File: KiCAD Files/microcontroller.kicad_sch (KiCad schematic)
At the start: 49 parts, among them IC5 AZ1117IH-3.3TRG1, J3 TSW-103-14-S-D, J4 TSW-103-14-S-D, J7 TSW-105-05-F-S, U1 STM32H7A3RGTx, Y1 ABM8G-48.000MHZ-18-D2Y-T

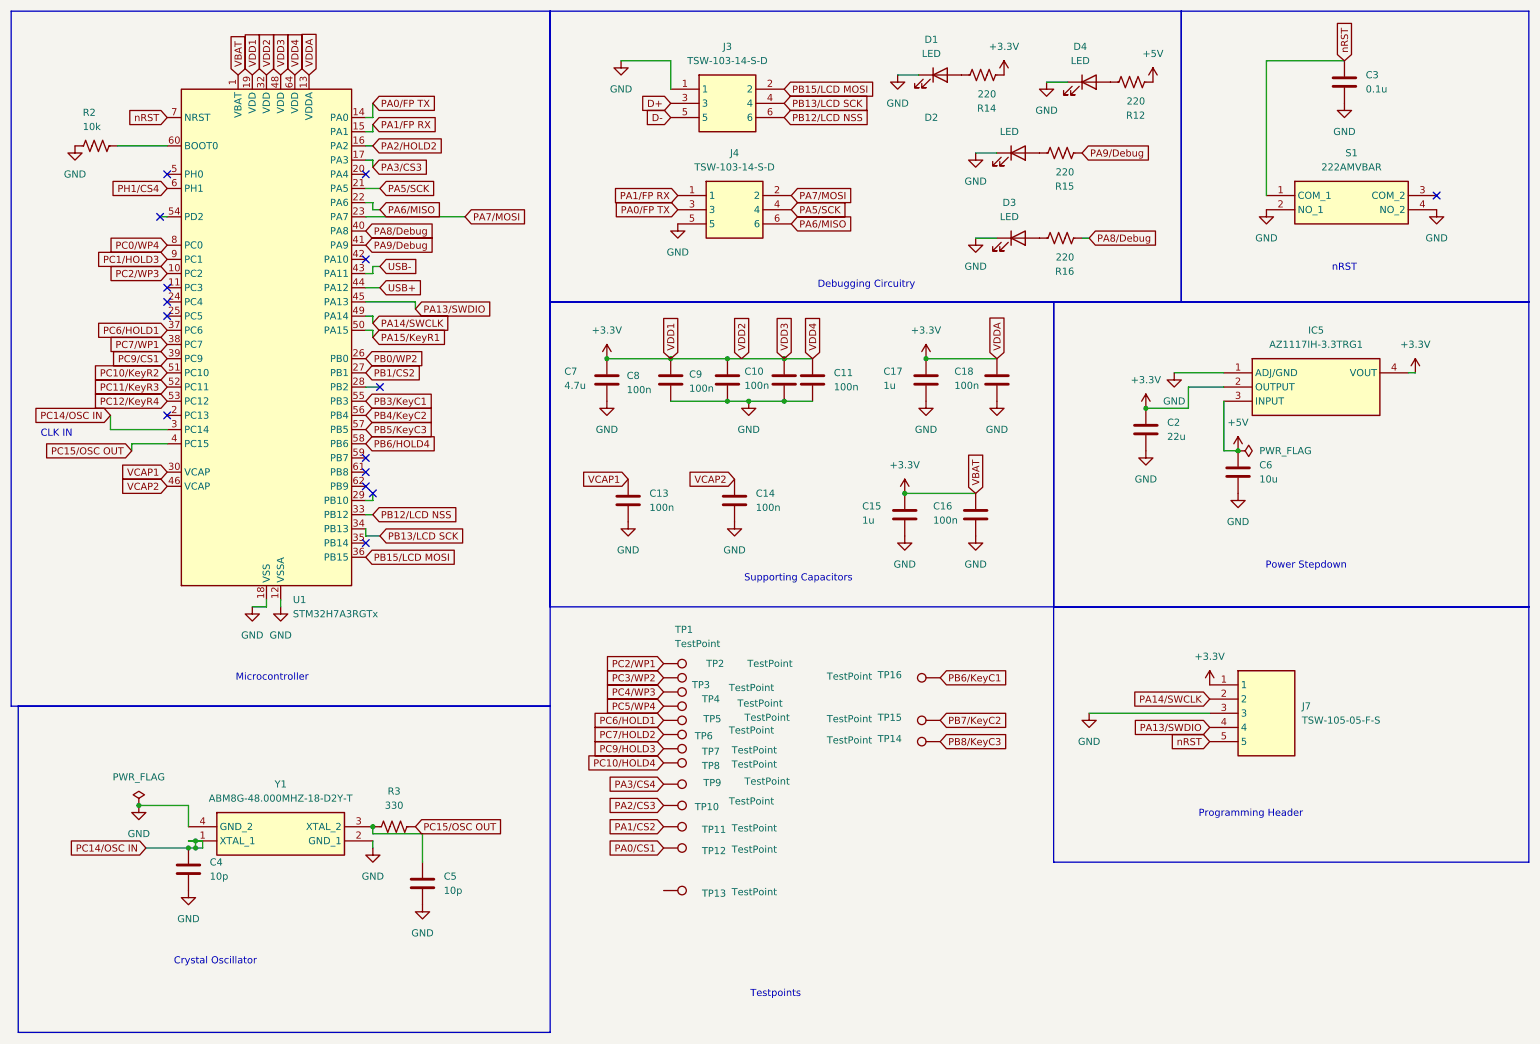
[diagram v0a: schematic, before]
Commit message: finalized 99% of pcb
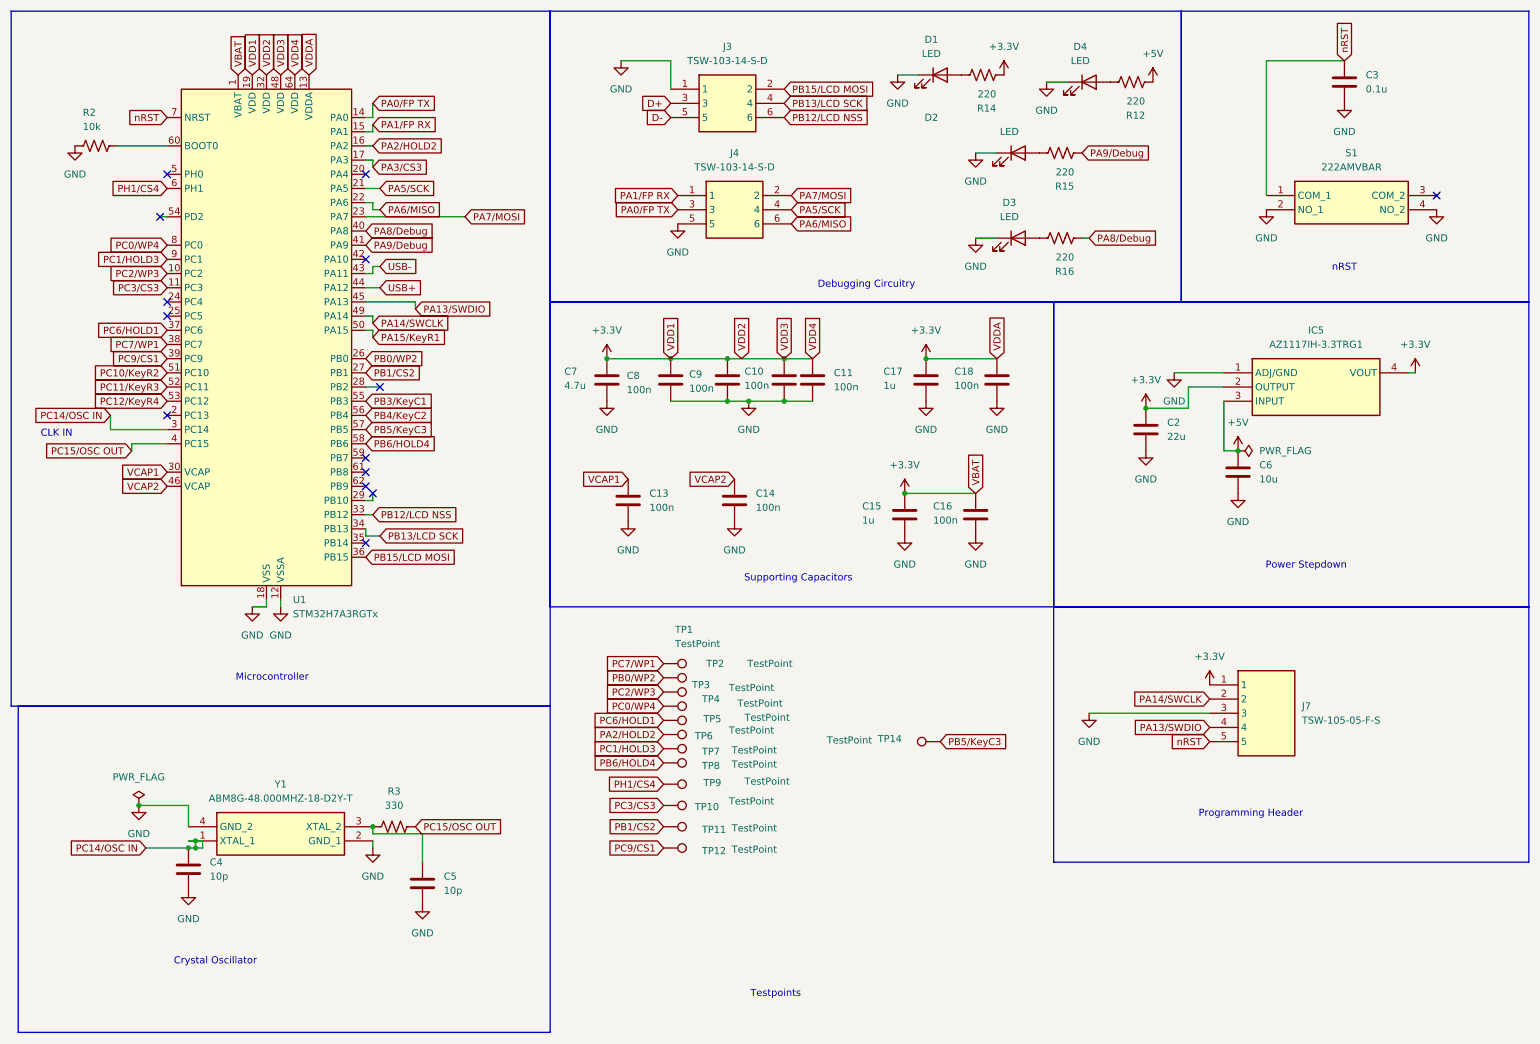
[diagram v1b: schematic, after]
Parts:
- removed TP13, TP15, TP16: TestPoint, TestPoint:TestPoint_THTPad_D1.5mm_Drill0.7mm, symbol Connector:TestPoint
- TP1, TP10, TP11, TP12, TP14, TP2, TP3, TP4, TP5, TP6, TP7, TP8, TP9: footprint TestPoint:TestPoint_THTPad_D1.5mm_Drill0.7mm -> TestPoint:TestPoint_THTPad_D1.0mm_Drill0.5mm
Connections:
- net PA0/CS1 is gone; now on net PC9/CS1: TP12.1
- net PA1/CS2 is gone; now on net PB1/CS2: TP11.1
- net PA2/CS3 is gone; now on net PC3/CS3: TP10.1
- net PA3/CS4 is gone; now on net PH1/CS4: TP9.1
- net PB8/KeyC3 is gone; now on net PB5/KeyC3: TP14.1
- net PC10/HOLD4 is gone; now on net PB6/HOLD4: TP8.1
- net PC2/WP1 is gone; now on net PC7/WP1: TP1.1
- net PC3/WP2 is gone; now on net PB0/WP2: TP2.1
- net PC4/WP3 is gone; now on net PC2/WP3: TP3.1
- net PC5/WP4 is gone; now on net PC0/WP4: TP4.1
- net PC7/HOLD2 is gone; now on net PA2/HOLD2: TP6.1
- net PC9/HOLD3 is gone; now on net PC1/HOLD3: TP7.1
- net PC3/CS3: now reaches U1.11 (PC3)
- no-connect marks 15 -> 14

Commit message: updated files with 3d models
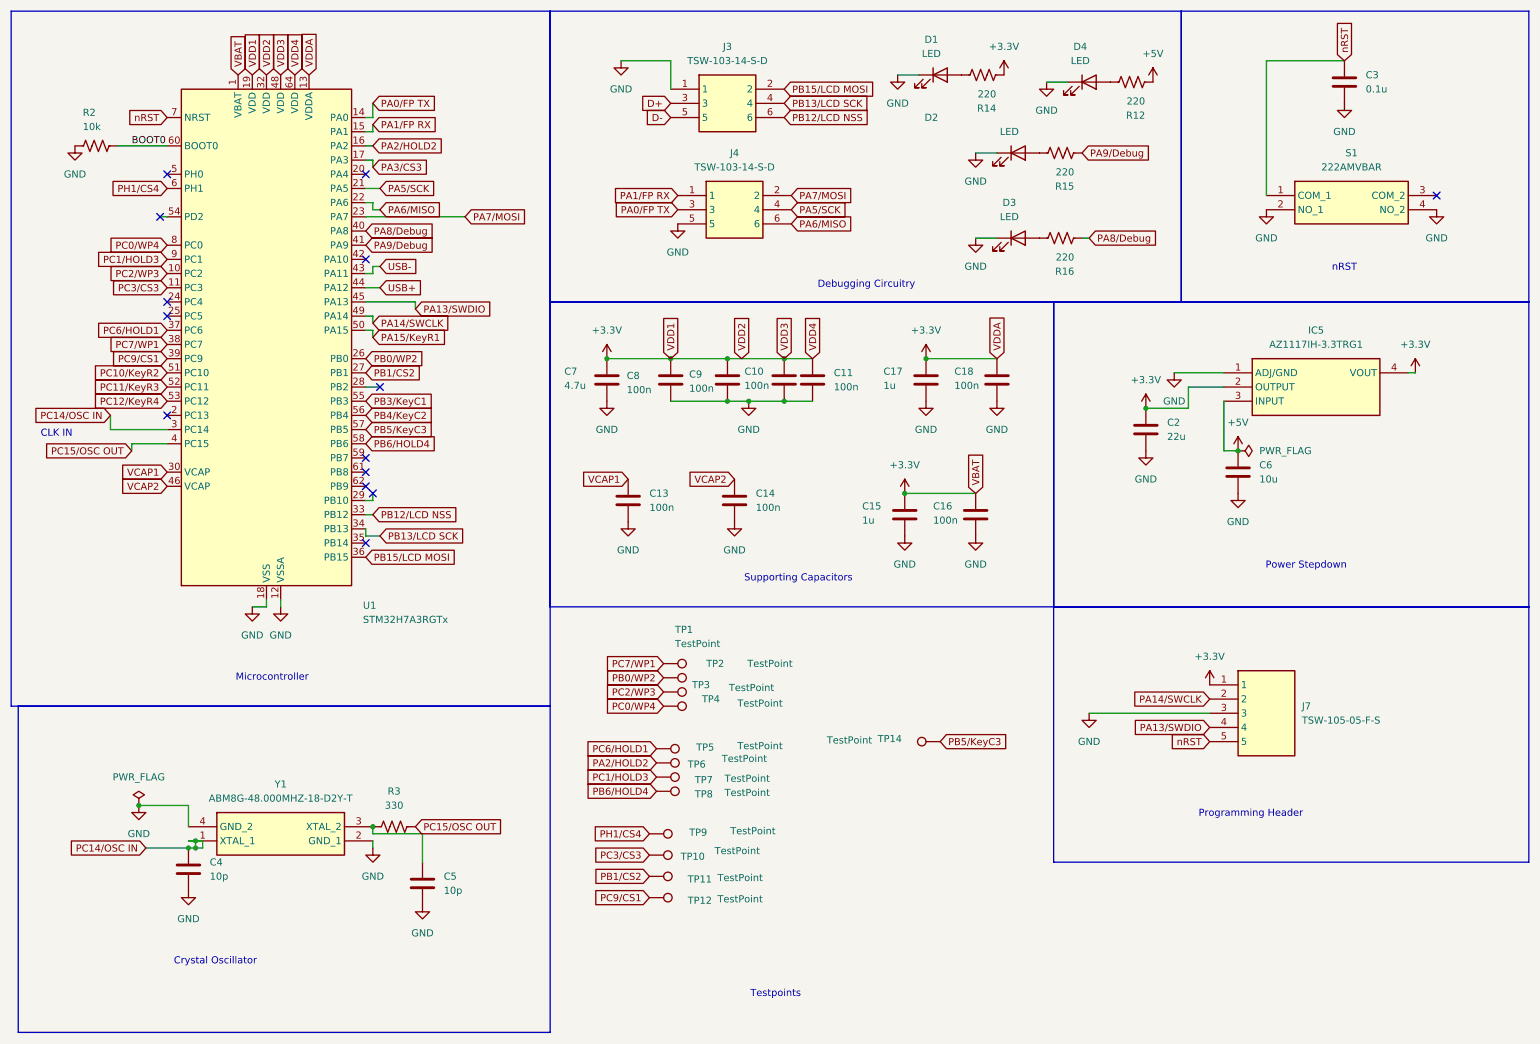
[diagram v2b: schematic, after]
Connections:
- net BOOT0: now reaches R2.1, U1.60 (BOOT0)
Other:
- moved on the sheet: TP10, TP11, TP12, TP5, TP6, TP7, TP8, TP9
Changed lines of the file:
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@@
 		)
 	)
+	(label "BOOT0"
+		(at 34.29 36.83 0)
+		(effects
+			(font
+				(size 1.27 1.27)
+			)
+			(justify left bottom)
+		)
+	)
 	(global_label "PC6{slash}HOLD1"
 		(shape input)
@@
 	(global_label "PC6{slash}HOLD1"
 		(shape input)
-		(at 129.54 139.7 180)
+		(at 128.27 144.78 180)
 		(fields_autoplaced yes)
 		(effects
@@
 		)
 		(property "Intersheetrefs" "${INTERSHEET_REFS}"
-			(at 115.3062 139.7 0)
+			(at 114.0362 144.78 0)
 			(effects
 				(font
@@
 	(global_label "PB1{slash}CS2"
 		(shape input)
-		(at 129.54 158.75 180)
+		(at 127 167.64 180)
 		(fields_autoplaced yes)
 		(effects
@@
 		)
 		(property "Intersheetrefs" "${INTERSHEET_REFS}"
-			(at 117.7858 158.75 0)
+			(at 115.2458 167.64 0)
 			(effects
 				(font
@@
 	(global_label "PH1{slash}CS4"
 		(shape input)
-		(at 129.54 151.13 180)
+		(at 127 160.02 180)
 		(fields_autoplaced yes)
 		(effects
@@
 		)
 		(property "Intersheetrefs" "${INTERSHEET_REFS}"
-			(at 117.7253 151.13 0)
+			(at 115.1853 160.02 0)
 			(effects
 				(font
@@
 	(global_label "PC1{slash}HOLD3"
 		(shape input)
-		(at 129.54 144.78 180)
+		(at 128.27 149.86 180)
 		(fields_autoplaced yes)
 		(effects
@@
 		)
 		(property "Intersheetrefs" "${INTERSHEET_REFS}"
-			(at 115.3062 144.78 0)
+			(at 114.0362 149.86 0)
 			(effects
 				(font
@@
 	(global_label "PB6{slash}HOLD4"
 		(shape input)
-		(at 129.54 147.32 180)
+		(at 128.27 152.4 180)
 		(fields_autoplaced yes)
 		(effects
@@
 		)
 		(property "Intersheetrefs" "${INTERSHEET_REFS}"
-			(at 115.3062 147.32 0)
+			(at 114.0362 152.4 0)
 			(effects
 				(font
@@
 	(global_label "PA2{slash}HOLD2"
 		(shape input)
-		(at 129.54 142.24 180)
+		(at 128.27 147.32 180)
 		(fields_autoplaced yes)
 		(effects
@@
 		)
 		(property "Intersheetrefs" "${INTERSHEET_REFS}"
-			(at 115.4876 142.24 0)
+			(at 114.2176 147.32 0)
 			(effects
 				(font
@@
 	(global_label "PC9{slash}CS1"
 		(shape input)
-		(at 129.54 162.56 180)
+		(at 127 171.45 180)
 		(fields_autoplaced yes)
 		(effects
@@
 		)
 		(property "Intersheetrefs" "${INTERSHEET_REFS}"
-			(at 117.7858 162.56 0)
+			(at 115.2458 171.45 0)
 			(effects
 				(font
@@
 	(global_label "PC3{slash}CS3"
 		(shape input)
-		(at 129.54 154.94 180)
+		(at 127 163.83 180)
 		(fields_autoplaced yes)
 		(effects
@@
 		)
 		(property "Intersheetrefs" "${INTERSHEET_REFS}"
-			(at 117.7858 154.94 0)
+			(at 115.2458 163.83 0)
 			(effects
 				(font
@@
 	(symbol
 		(lib_id "Connector:TestPoint")
-		(at 129.54 147.32 270)
+		(at 128.27 152.4 270)
 		(unit 1)
 		(exclude_from_sim no)
@@
 		(dnp no)
 		(property "Reference" "TP8"
-			(at 136.398 147.828 90)
+			(at 135.128 152.908 90)
 			(effects
 				(font
@@
 		)
 		(property "Value" "TestPoint"
-			(at 141.732 147.574 90)
+			(at 140.462 152.654 90)
 			(effects
 				(font
@@
 		)
 		(property "Footprint" "TestPoint:TestPoint_THTPad_D1.0mm_Drill0.5mm"
-			(at 129.54 152.4 0)
+			(at 128.27 157.48 0)
 			(effects
 				(font
@@
 		)
 		(property "Datasheet" "~"
-			(at 129.54 152.4 0)
+			(at 128.27 157.48 0)
 			(effects
 				(font
@@
 		)
 		(property "Description" "test point"
-			(at 129.54 147.32 0)
+			(at 128.27 152.4 0)
 			(effects
 				(font
@@
 	(symbol
 		(lib_id "Connector:TestPoint")
-		(at 129.54 142.24 270)
+		(at 128.27 147.32 270)
 		(unit 1)
 		(exclude_from_sim no)
@@
 		(dnp no)
 		(property "Reference" "TP6"
-			(at 135.128 142.494 90)
+			(at 133.858 147.574 90)
 			(effects
 				(font
@@
 		)
 		(property "Value" "TestPoint"
-			(at 141.224 141.478 90)
+			(at 139.954 146.558 90)
 			(effects
 				(font
@@
 		)
 		(property "Footprint" "TestPoint:TestPoint_THTPad_D1.0mm_Drill0.5mm"
-			(at 129.54 147.32 0)
+			(at 128.27 152.4 0)
 			(effects
 				(font
@@
 		)
 		(property "Datasheet" "~"
-			(at 129.54 147.32 0)
+			(at 128.27 152.4 0)
 			(effects
 				(font
@@
 		)
 		(property "Description" "test point"
-			(at 129.54 142.24 0)
+			(at 128.27 147.32 0)
 			(effects
 				(font
@@
 	(symbol
 		(lib_id "Connector:TestPoint")
-		(at 129.54 154.94 270)
+		(at 127 163.83 270)
 		(unit 1)
 		(exclude_from_sim no)
@@
 		(dnp no)
 		(property "Reference" "TP10"
-			(at 135.128 155.194 90)
+			(at 132.588 164.084 90)
 			(effects
 				(font
@@
 		)
 		(property "Value" "TestPoint"
-			(at 141.224 154.178 90)
+			(at 138.684 163.068 90)
 			(effects
 				(font
@@
 		)
 		(property "Footprint" "TestPoint:TestPoint_THTPad_D1.0mm_Drill0.5mm"
-			(at 129.54 160.02 0)
+			(at 127 168.91 0)
 			(effects
 				(font
@@
 		)
 		(property "Datasheet" "~"
-			(at 129.54 160.02 0)
+			(at 127 168.91 0)
 			(effects
 				(font
@@
 		)
 		(property "Description" "test point"
-			(at 129.54 154.94 0)
+			(at 127 163.83 0)
 			(effects
 				(font
@@
 	(symbol
 		(lib_id "Connector:TestPoint")
-		(at 129.54 162.56 270)
+		(at 127 171.45 270)
 		(unit 1)
 		(exclude_from_sim no)
@@
 		(dnp no)
 		(property "Reference" "TP12"
-			(at 136.398 163.068 90)
+			(at 133.858 171.958 90)
 			(effects
 				(font
@@
 		)
 		(property "Value" "TestPoint"
-			(at 141.732 162.814 90)
+			(at 139.192 171.704 90)
 			(effects
 				(font
@@
 		)
 		(property "Footprint" "TestPoint:TestPoint_THTPad_D1.0mm_Drill0.5mm"
-			(at 129.54 167.64 0)
+			(at 127 176.53 0)
 			(effects
 				(font
@@
 		)
 		(property "Datasheet" "~"
-			(at 129.54 167.64 0)
+			(at 127 176.53 0)
 			(effects
 				(font
@@
 		)
 		(property "Description" "test point"
-			(at 129.54 162.56 0)
+			(at 127 171.45 0)
 			(effects
 				(font
@@
 	(symbol
 		(lib_id "Connector:TestPoint")
-		(at 129.54 139.7 270)
+		(at 128.27 144.78 270)
 		(unit 1)
 		(exclude_from_sim no)
@@
 		(dnp no)
 		(property "Reference" "TP5"
-			(at 136.652 139.446 90)
+			(at 135.382 144.526 90)
 			(effects
 				(font
@@
 		)
 		(property "Value" "TestPoint"
-			(at 144.018 139.192 90)
+			(at 142.748 144.272 90)
 			(effects
 				(font
@@
 		)
 		(property "Footprint" "TestPoint:TestPoint_THTPad_D1.0mm_Drill0.5mm"
-			(at 129.54 144.78 0)
+			(at 128.27 149.86 0)
 			(effects
 				(font
@@
 		)
 		(property "Datasheet" "~"
-			(at 129.54 144.78 0)
+			(at 128.27 149.86 0)
 			(effects
 				(font
@@
 		)
 		(property "Description" "test point"
-			(at 129.54 139.7 0)
+			(at 128.27 144.78 0)
 			(effects
 				(font
@@
 	(symbol
 		(lib_id "Connector:TestPoint")
-		(at 129.54 151.13 270)
+		(at 127 160.02 270)
 		(unit 1)
 		(exclude_from_sim no)
@@
 		(dnp no)
 		(property "Reference" "TP9"
-			(at 136.652 150.876 90)
+			(at 134.112 159.766 90)
 			(effects
 				(font
@@
 		)
 		(property "Value" "TestPoint"
-			(at 144.018 150.622 90)
+			(at 141.478 159.512 90)
 			(effects
 				(font
@@
 		)
 		(property "Footprint" "TestPoint:TestPoint_THTPad_D1.0mm_Drill0.5mm"
-			(at 129.54 156.21 0)
+			(at 127 165.1 0)
 			(effects
 				(font
@@
 		)
 		(property "Datasheet" "~"
-			(at 129.54 156.21 0)
+			(at 127 165.1 0)
 			(effects
 				(font
@@
 		)
 		(property "Description" "test point"
-			(at 129.54 151.13 0)
+			(at 127 160.02 0)
 			(effects
 				(font
@@
 		(on_board yes)
 		(dnp no)
-		(fields_autoplaced yes)
 		(property "Reference" "U1"
-			(at 63.1541 118.11 0)
+			(at 75.692 119.126 0)
 			(effects
 				(font
@@
 		)
 		(property "Value" "STM32H7A3RGTx"
-			(at 63.1541 120.65 0)
+			(at 75.692 121.666 0)
 			(effects
 				(font
@@
 	(symbol
 		(lib_id "Connector:TestPoint")
-		(at 129.54 158.75 270)
+		(at 127 167.64 270)
 		(unit 1)
 		(exclude_from_sim no)
@@
 		(dnp no)
 		(property "Reference" "TP11"
-			(at 136.398 159.258 90)
+			(at 133.858 168.148 90)
 			(effects
 				(font
@@
 		)
 		(property "Value" "TestPoint"
-			(at 141.732 159.004 90)
+			(at 139.192 167.894 90)
 			(effects
 				(font
@@
 		)
 		(property "Footprint" "TestPoint:TestPoint_THTPad_D1.0mm_Drill0.5mm"
-			(at 129.54 163.83 0)
+			(at 127 172.72 0)
 			(effects
 				(font
@@
 		)
 		(property "Datasheet" "~"
-			(at 129.54 163.83 0)
+			(at 127 172.72 0)
 			(effects
 				(font
@@
 		)
 		(property "Description" "test point"
-			(at 129.54 158.75 0)
+			(at 127 167.64 0)
 			(effects
 				(font
@@
 	(symbol
 		(lib_id "Connector:TestPoint")
-		(at 129.54 144.78 270)
+		(at 128.27 149.86 270)
 		(unit 1)
 		(exclude_from_sim no)
@@
 		(dnp no)
 		(property "Reference" "TP7"
-			(at 136.398 145.288 90)
+			(at 135.128 150.368 90)
 			(effects
 				(font
@@
 		)
 		(property "Value" "TestPoint"
-			(at 141.732 145.034 90)
+			(at 140.462 150.114 90)
 			(effects
 				(font
@@
 		)
 		(property "Footprint" "TestPoint:TestPoint_THTPad_D1.0mm_Drill0.5mm"
-			(at 129.54 149.86 0)
+			(at 128.27 154.94 0)
 			(effects
 				(font
@@
 		)
 		(property "Datasheet" "~"
-			(at 129.54 149.86 0)
+			(at 128.27 154.94 0)
 			(effects
 				(font
@@
 		)
 		(property "Description" "test point"
-			(at 129.54 144.78 0)
+			(at 128.27 149.86 0)
 			(effects
 				(font
